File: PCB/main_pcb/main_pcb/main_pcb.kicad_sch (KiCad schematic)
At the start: 52 parts, among them J1 Conn_01x20_Socket, J2 Conn_01x20_Socket, J3 Conn_01x09_Socket, Q1 DMG2305UX-7, SW0_Header1 B6B-XH-A, SW1_Header1 B6B-XH-A

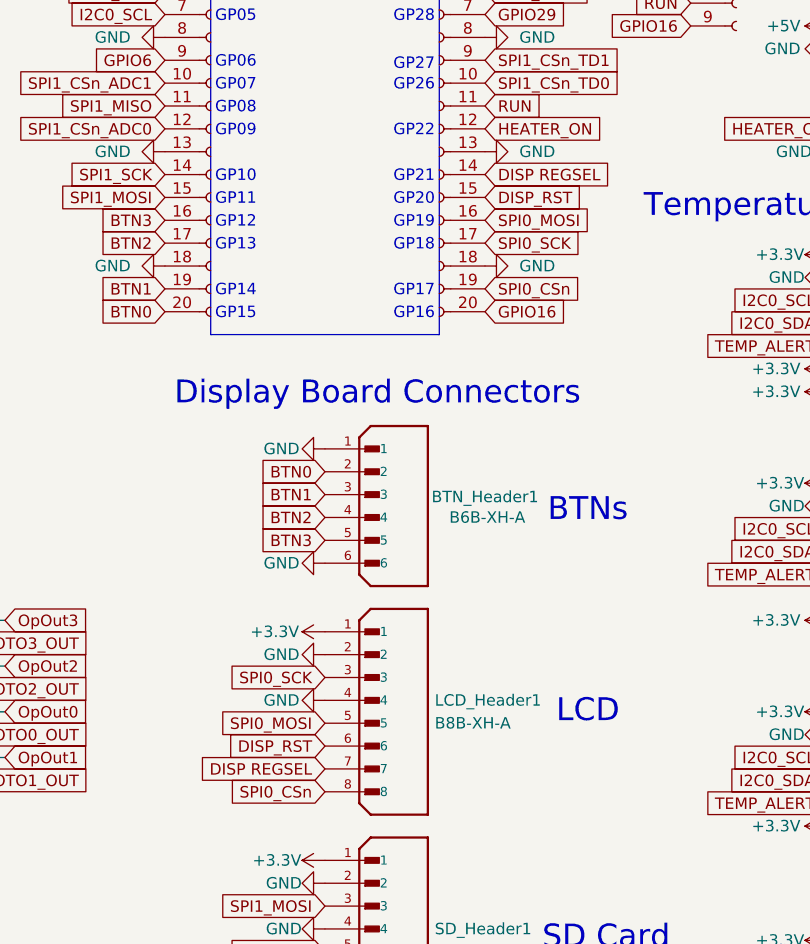
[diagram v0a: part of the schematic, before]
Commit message: A lot of changes, display logic and some error handling
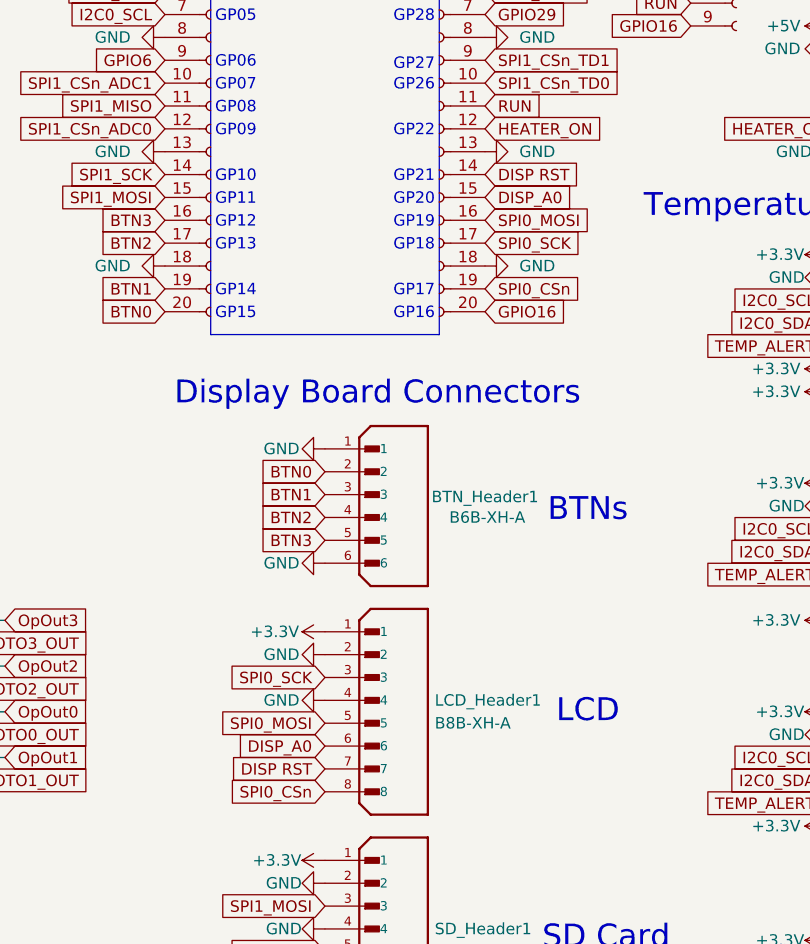
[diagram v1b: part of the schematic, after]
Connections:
- net DISP REGSEL renamed DISP RST
- net DISP_RST renamed DISP_A0
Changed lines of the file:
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@@
 		)
 	)
-	(global_label "DISP REGSEL"
+	(global_label "DISP RST"
 		(shape input)
 		(at 330.2 52.07 0)
@@
 		)
 		(property "Intersheetrefs" "${INTERSHEET_REFS}"
-			(at 345.5827 52.07 0)
+			(at 341.9542 52.07 0)
 			(effects
 				(font
@@
 		)
 	)
-	(global_label "DISP REGSEL"
+	(global_label "DISP RST"
 		(shape input)
 		(at 312.42 118.11 180)
@@
 		)
 		(property "Intersheetrefs" "${INTERSHEET_REFS}"
-			(at 297.0373 118.11 0)
+			(at 300.6658 118.11 0)
 			(effects
 				(font
@@
 		)
 	)
-	(global_label "DISP_RST"
+	(global_label "DISP_A0"
 		(shape input)
 		(at 330.2 54.61 0)
@@
 		)
 		(property "Intersheetrefs" "${INTERSHEET_REFS}"
-			(at 341.9542 54.61 0)
+			(at 340.8052 54.61 0)
 			(effects
 				(font
@@
 		)
 	)
-	(global_label "DISP_RST"
+	(global_label "DISP_A0"
 		(shape input)
 		(at 312.42 115.57 180)
@@
 		)
 		(property "Intersheetrefs" "${INTERSHEET_REFS}"
-			(at 300.6658 115.57 0)
-			(effects
-				(font
+			(at 301.8148 115.57 0)
+			(effects
+				(font
